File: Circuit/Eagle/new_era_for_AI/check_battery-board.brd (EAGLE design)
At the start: 94 x 70 mm, 32 parts

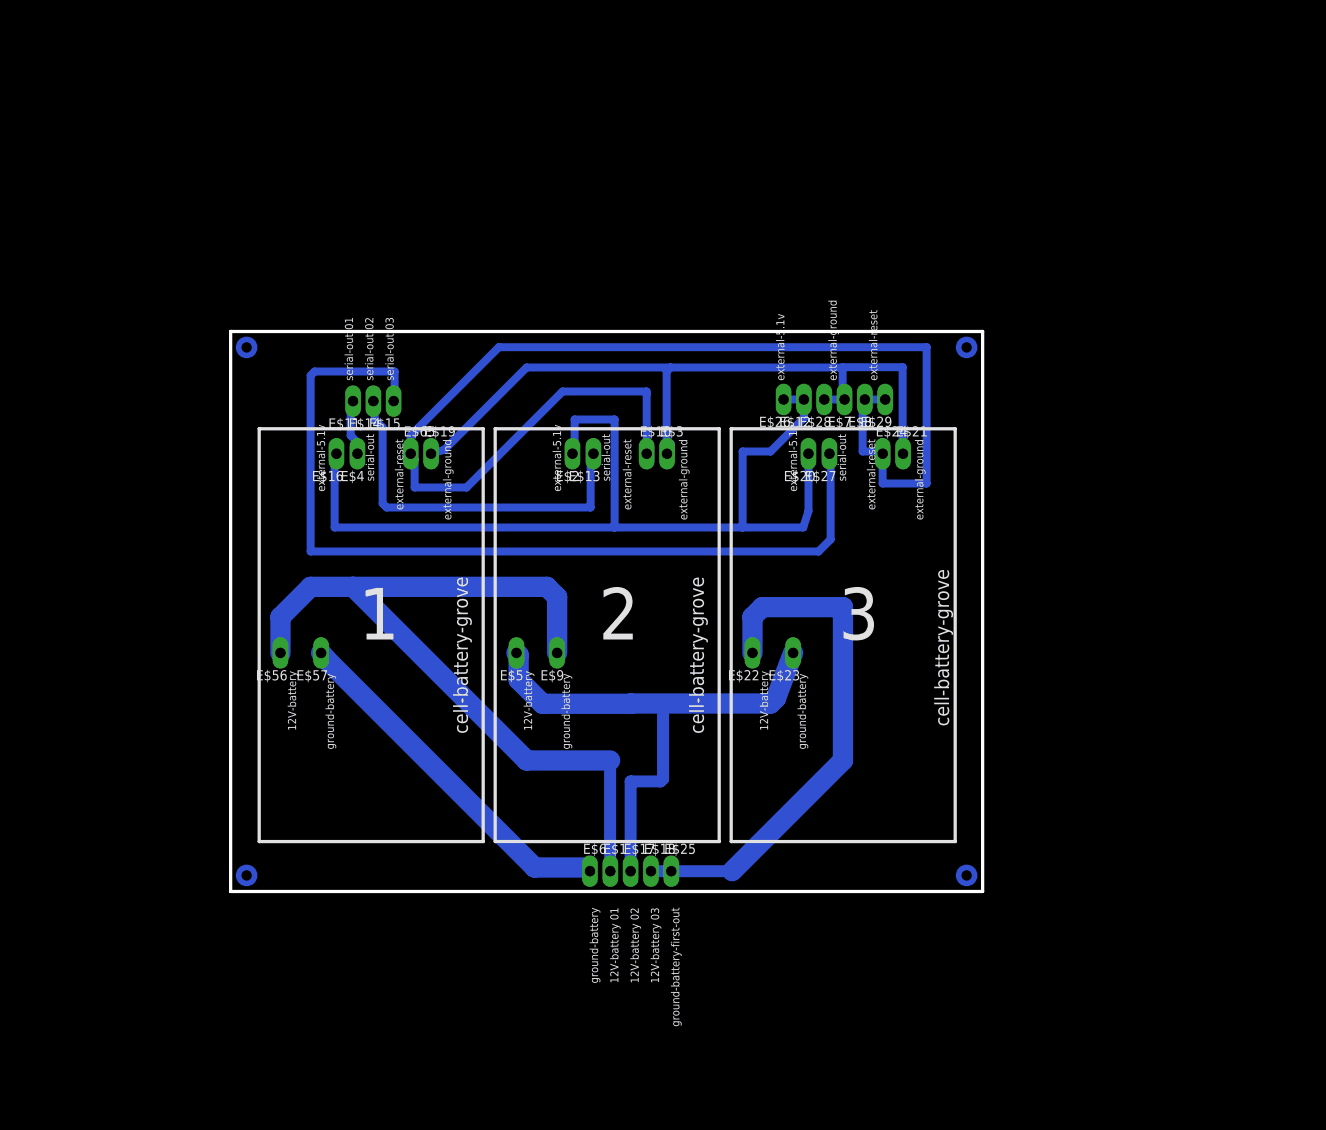
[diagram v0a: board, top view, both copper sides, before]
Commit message: .
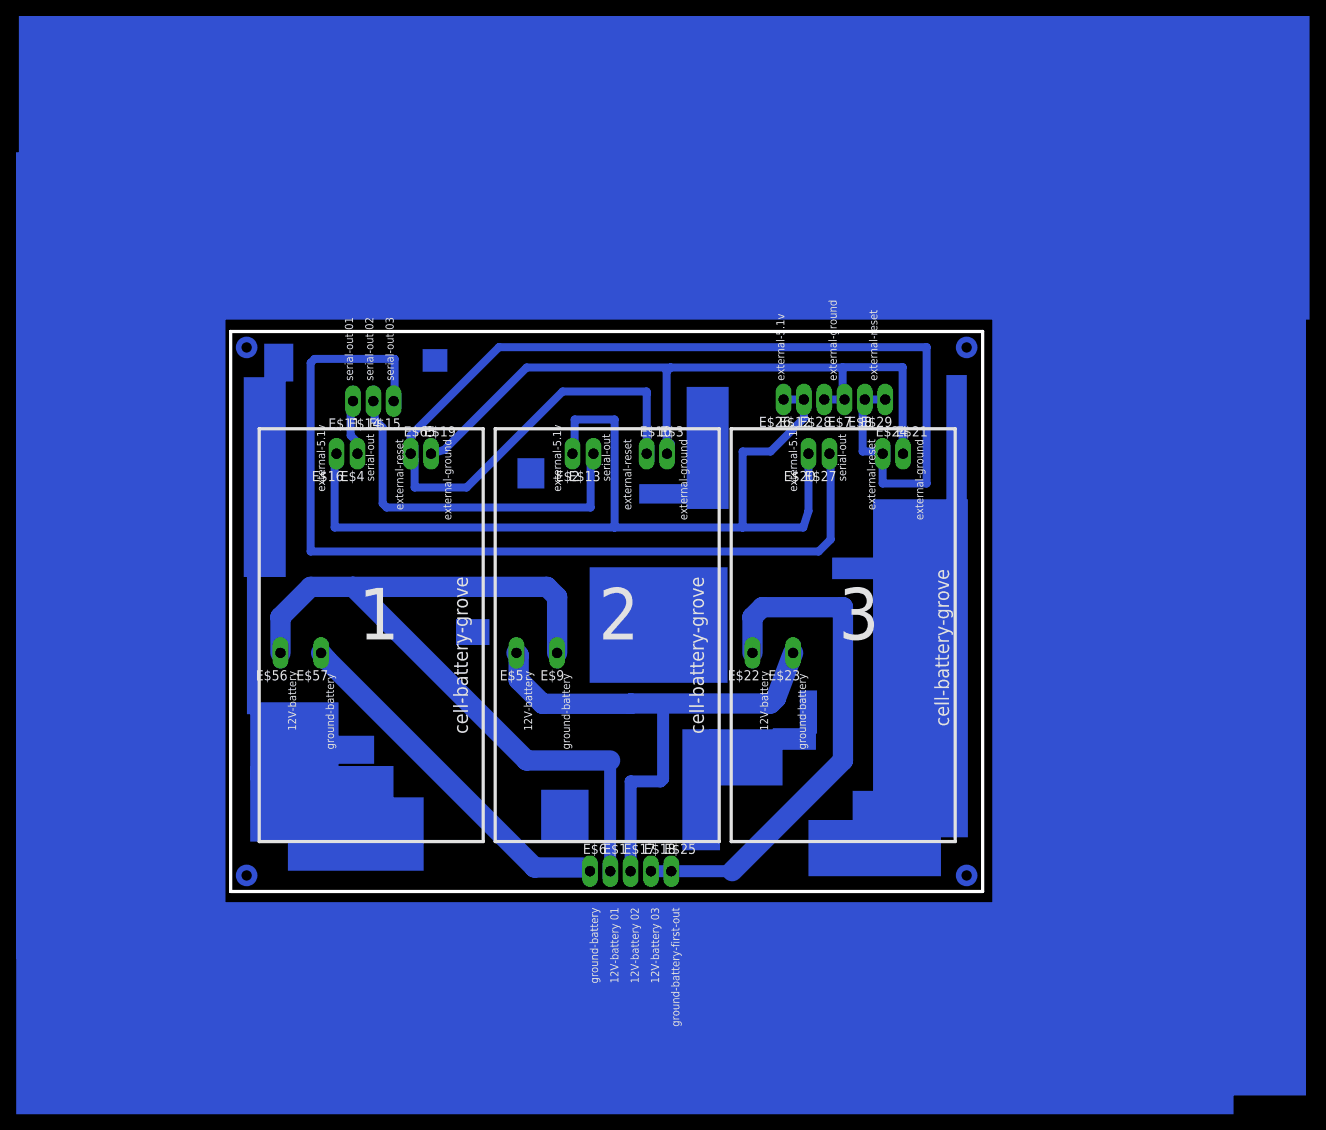
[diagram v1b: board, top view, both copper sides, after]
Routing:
- net S$11: track 112.8 -> 116.0 mm
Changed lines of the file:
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@@
 <layer number="19" name="Unrouted" color="6" fill="1" visible="yes" active="yes"/>
 <layer number="20" name="Dimension" color="15" fill="1" visible="yes" active="yes"/>
-<layer number="21" name="tPlace" color="7" fill="1" visible="yes" active="yes"/>
+<layer number="21" name="tPlace" color="7" fill="1" visible="no" active="yes"/>
 <layer number="22" name="bPlace" color="7" fill="1" visible="no" active="yes"/>
 <layer number="23" name="tOrigins" color="15" fill="1" visible="no" active="yes"/>
 <layer number="24" name="bOrigins" color="15" fill="1" visible="no" active="yes"/>
 <layer number="25" name="tNames" color="7" fill="1" visible="no" active="yes"/>
-<layer number="26" name="bNames" color="7" fill="1" visible="yes" active="yes"/>
+<layer number="26" name="bNames" color="7" fill="1" visible="no" active="yes"/>
 <layer number="27" name="tValues" color="7" fill="1" visible="no" active="yes"/>
 <layer number="28" name="bValues" color="7" fill="1" visible="no" active="yes"/>
@@
 <layer number="45" name="Holes" color="7" fill="1" visible="yes" active="yes"/>
 <layer number="46" name="Milling" color="3" fill="1" visible="no" active="yes"/>
-<layer number="47" name="Measures" color="7" fill="1" visible="yes" active="yes"/>
+<layer number="47" name="Measures" color="7" fill="1" visible="no" active="yes"/>
 <layer number="48" name="Document" color="7" fill="1" visible="no" active="yes"/>
 <layer number="49" name="Reference" color="7" fill="1" visible="no" active="yes"/>
@@
 <wire x1="2" y1="72" x2="96" y2="72" width="0.4064" layer="20"/>
 <wire x1="96" y1="2" x2="2" y2="2" width="0.4064" layer="20"/>
-<dimension x1="2" y1="72" x2="96" y2="72" x3="49" y3="86" textsize="1.778" layer="20"/>
-<dimension x1="2" y1="2" x2="2" y2="72" x3="-8" y3="37" textsize="1.778" layer="20"/>
+<dimension x1="2" y1="72" x2="96" y2="72" x3="49" y3="86" textsize="1.778" layer="47"/>
+<dimension x1="2" y1="2" x2="2" y2="72" x3="-8" y3="37" textsize="1.778" layer="47"/>
 <text x="57.08" y="0" size="1.016" layer="21" rot="R270">ground-battery-first-out</text>
 <wire x1="2.001834375" y1="2.008475" x2="2.001834375" y2="72.008475" width="0.4064" layer="20"/>
@@
 <circle x="4.001834375" y="4.008475" radius="1" width="0.7" layer="16"/>
 <circle x="94.001834375" y="4.008475" radius="1" width="0.7" layer="16"/>
+<rectangle x1="9.159853125" y1="4.59029375" x2="26.13251875" y2="13.770884375" layer="16"/>
+<rectangle x1="4.445221875" y1="8.235528125" x2="22.360815625" y2="17.686134375" layer="16"/>
+<rectangle x1="5.522853125" y1="17.956153125" x2="19.936146875" y2="21.466378125" layer="16"/>
+<rectangle x1="4.445221875" y1="15.931021875" x2="15.490925" y2="25.651646875" layer="16"/>
+<rectangle x1="74.221740625" y1="3.91525" x2="90.790296875" y2="10.9357" layer="16"/>
+<rectangle x1="79.879296875" y1="4.455284375" x2="84.9980375" y2="8.3705375" layer="16"/>
+<rectangle x1="82.3039625" y1="8.7755625" x2="94.1578875" y2="51.033275" layer="16"/>
+<rectangle x1="3.637" y1="41.31265" x2="8.89044375" y2="66.289253125" layer="16"/>
+<rectangle x1="46.8768875" y1="28.0818" x2="64.1189625" y2="42.527728125" layer="16"/>
+<rectangle x1="58.596109375" y1="7.29046875" x2="60.4819625" y2="11.745753125" layer="16"/>
+<rectangle x1="58.46140625" y1="7.155459375" x2="63.1760375" y2="22.276428125" layer="16"/>
+<rectangle x1="61.829" y1="15.255978125" x2="70.988853125" y2="22.276428125" layer="16"/>
+<rectangle x1="69.77651875" y1="19.711265625" x2="75.164665625" y2="22.4114375" layer="16"/>
+<rectangle x1="73.144109375" y1="21.73639375" x2="75.29936875" y2="27.136740625" layer="16"/>
+<rectangle x1="37.851740625" y1="52.383359375" x2="41.219334375" y2="56.163603125" layer="16"/>
+<rectangle x1="59.000221875" y1="49.818196875" x2="64.253665625" y2="65.074175" layer="16"/>
+<rectangle x1="53.073259375" y1="50.4932375" x2="60.75136875" y2="52.92339375" layer="16"/>
+<rectangle x1="4.0411125" y1="24.16655" x2="5.65755625" y2="43.607796875" layer="16"/>
+<rectangle x1="30.173628125" y1="32.807103125" x2="34.34944375" y2="36.0473125" layer="16"/>
+<rectangle x1="40.815221875" y1="8.3705375" x2="46.742184375" y2="14.71594375" layer="16"/>
+<rectangle x1="77.185221875" y1="41.04263125" x2="84.055109375" y2="43.74280625" layer="16"/>
+<rectangle x1="79.74459375" y1="9.315596875" x2="83.651" y2="14.580934375" layer="16"/>
+<rectangle x1="91.463815625" y1="49.953203125" x2="94.023184375" y2="66.55926875" layer="16"/>
+<rectangle x1="25.997815625" y1="66.964296875" x2="29.096" y2="69.799478125" layer="16"/>
+<rectangle x1="6.196371875" y1="65.74921875" x2="9.833371875" y2="70.474521875" layer="16"/>
+<rectangle x1="-24.8285875" y1="-6.41004375" x2="1.3578125" y2="94.402484375" layer="16"/>
+<rectangle x1="-24.80375625" y1="-25.845303125" x2="127.37064375" y2="0.67130625" layer="16"/>
+<rectangle x1="97.2039125" y1="-23.495728125" x2="136.420665625" y2="98.34640625" layer="16"/>
+<rectangle x1="-24.468571875" y1="73.481246875" x2="136.86758125" y2="111.436884375" layer="16"/>
 </plain>
 <attributes>
@@
 <contactref element="E$15" pad="TP"/>
 <contactref element="E$27" pad="TP"/>
-<wire x1="22.5" y1="67" x2="22.5" y2="63.42" width="1" layer="16"/>
+<wire x1="22.5" y1="68.57340625" x2="22.5" y2="63.42" width="1" layer="16"/>
 <wire x1="22.38" y1="63.3" x2="22.5" y2="63.42" width="1" layer="16"/>
-<wire x1="12.5" y1="67" x2="22.5" y2="67" width="1" layer="16"/>
-<wire x1="12" y1="66.5" x2="12.5" y2="67" width="1" layer="16"/>
-<wire x1="12" y1="44.5" x2="12" y2="66.5" width="1" layer="16"/>
+<wire x1="12.501196875" y1="68.57340625" x2="22.5" y2="68.57340625" width="1" layer="16"/>
+<wire x1="12" y1="68.072209375" x2="12.501196875" y2="68.57340625" width="1" layer="16"/>
+<wire x1="12" y1="44.5" x2="12" y2="68.072209375" width="1" layer="16"/>
 <wire x1="75.5" y1="44.5" x2="12" y2="44.5" width="1" layer="16"/>
 <wire x1="77" y1="46" x2="75.5" y2="44.5" width="1" layer="16"/>
